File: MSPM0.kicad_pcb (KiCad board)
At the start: 2 copper layers, 0 parts

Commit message: Positioned components, made schematic adjustment accordingly Created ground layer
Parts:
- added C1: 10u, Capacitor_SMD:C_0805_2012Metric, F.Cu at (61.0, 87.8)
- added C10: 10u, Capacitor_SMD:C_0805_2012Metric, F.Cu at (48.0, 80.1)
- added C11: 470n, Capacitor_SMD:C_0603_1608Metric, F.Cu at (51.3, 82.6)
- added C12: 470n, Capacitor_SMD:C_0603_1608Metric, F.Cu at (54.5, 86.1)
- added C13: 470n, Capacitor_SMD:C_0603_1608Metric, F.Cu at (54.5, 91.1)
- added C14: 470n, Capacitor_SMD:C_0603_1608Metric, F.Cu at (70.0, 98.1)
- added C2: 470n, Capacitor_SMD:C_0603_1608Metric, F.Cu at (64.0, 81.8)
- added C3: 470n, Capacitor_SMD:C_0603_1608Metric, F.Cu at (68.5, 81.6)
- added C4: 470n, Capacitor_SMD:C_0603_1608Metric, F.Cu at (76.0, 91.6)
- added C5: 15p, Capacitor_SMD:C_0603_1608Metric, F.Cu at (63.0, 94.9)
- added C6: 15p, Capacitor_SMD:C_0603_1608Metric, F.Cu at (57.0, 94.8)
- added C7: 470n, Capacitor_SMD:C_0603_1608Metric, F.Cu at (43.7, 82.1)
- added C8: 470n, Capacitor_SMD:C_0603_1608Metric, F.Cu at (45.2, 82.1)
- added C9: 10u, Capacitor_SMD:C_0805_2012Metric, F.Cu at (54.8, 80.1)
- added D1: USBLC6-2SC6, Package_TO_SOT_SMD:SOT-23-6, F.Cu at (44.7, 87.3)
- added FID1: Fiducial, Fiducial:Fiducial_1mm_Mask2mm, F.Cu at (42.2, 76.2)
- added FID2: Fiducial, Fiducial:Fiducial_1mm_Mask2mm, F.Cu at (89.9, 76.2)
- added FID3: Fiducial, Fiducial:Fiducial_1mm_Mask2mm, F.Cu at (89.9, 97.8)
- added J1: USB4105-GF-A, Connector_USB:USB_C_Receptacle_GCT_USB4105-xx-A_16P_TopMnt_Horizontal, F.Cu at (36.0, 86.4)
- added J2: TC2030, Connector:Tag-Connect_TC2030-IDC-FP_2x03_P1.27mm_Vertical, F.Cu at (81.5, 88.4)
- added MH1: M3, MountingHole:MountingHole_3.2mm_M3_Pad_Via, F.Cu at (95.2, 97.8)
- added MH2: M3, MountingHole:MountingHole_3.2mm_M3_Pad_Via, F.Cu at (95.2, 76.2)
- added MH3: M3, MountingHole:MountingHole_3.2mm_M3_Pad_Via, F.Cu at (36.8, 97.8)
- added MH4: M3, MountingHole:MountingHole_3.2mm_M3_Pad_Via, F.Cu at (36.8, 76.2)
- added R1: 0R, Capacitor_SMD:C_0603_1608Metric, F.Cu at (68.5, 80.1)
- added R2: 5k1, Capacitor_SMD:C_0603_1608Metric, F.Cu at (74.5, 91.6)
- added R3: 100k, Capacitor_SMD:C_0603_1608Metric, F.Cu at (60.5, 90.3)
- added R4: 0R, Capacitor_SMD:C_0603_1608Metric, F.Cu at (44.5, 84.3)
- added R5: 5k1, Capacitor_SMD:C_0603_1608Metric, F.Cu at (41.0, 92.6)
- added R6: 5k1, Capacitor_SMD:C_0603_1608Metric, F.Cu at (40.8, 79.8)
- added R7: 5k1, Capacitor_SMD:C_0603_1608Metric, F.Cu at (69.5, 95.6)
- added R8: 5k1, Capacitor_SMD:C_0603_1608Metric, F.Cu at (66.5, 95.6)
- added U1: MSPM0G3507SPTR, Package_QFP:LQFP-48_7x7mm_P0.5mm, F.Cu at (67.8, 88.1)
- added U2: SPX3819M5-L-3-3, Package_TO_SOT_SMD:SOT-23-5, F.Cu at (51.3, 80.1)
- added U3: CH340E, Package_SO:MSOP-10_3x3mm_P0.5mm, F.Cu at (54.5, 88.6)
- added U4: LIS2DH, Package_LGA:LGA-14_2x2mm_P0.35mm_LayoutBorder3x4y, F.Cu at (68.0, 98.1)
- added X1: 8MHz, Crystal:Crystal_SMD_3225-4Pin_3.2x2.5mm, F.Cu at (60.0, 94.8)
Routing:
- added copper zone on B.Cu, net GND
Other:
- board outline added: 66 x 29.2 mm

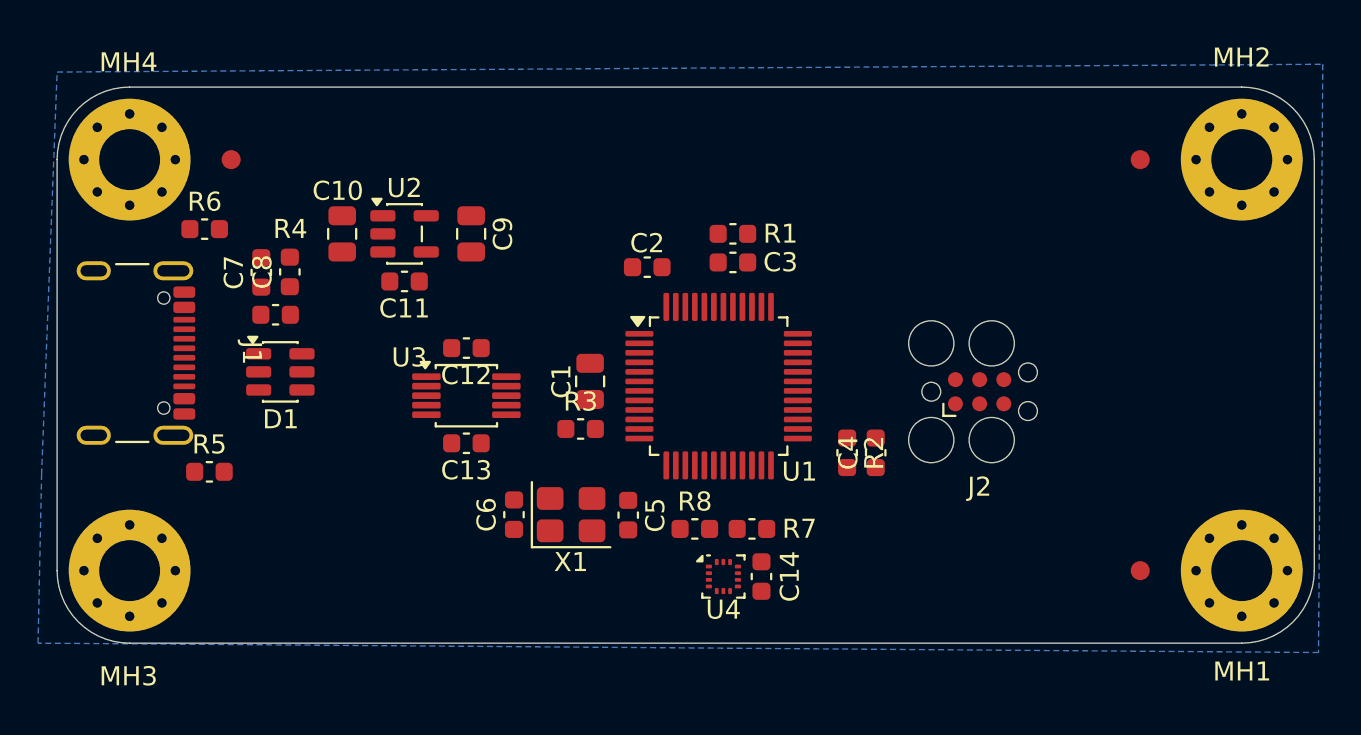
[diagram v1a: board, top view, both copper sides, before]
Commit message: Completed mk. I
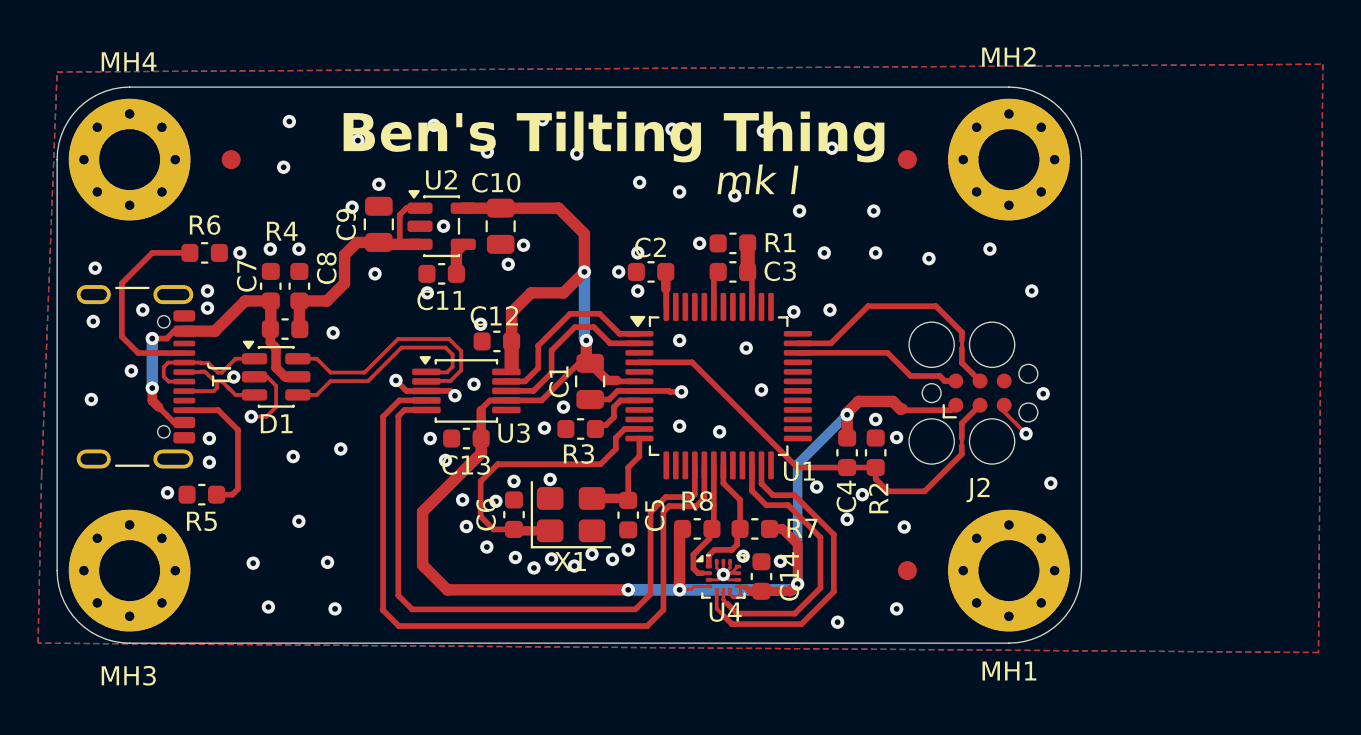
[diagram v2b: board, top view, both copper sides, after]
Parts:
- moved MH1 12.2 mm to (83.0, 97.8)
- moved MH2 12.2 mm to (83.0, 76.2)
- moved FID2 12.2 mm to (77.7, 76.2)
- moved FID3 12.2 mm to (77.7, 97.8)
- moved C10 8.33 mm to (56.3, 79.7)
- moved C9 4.88 mm to (49.9, 79.6), turned to 90 degrees
- moved C11 1.99 mm to (53.2, 82.2)
- moved U2 1.99 mm to (53.2, 79.7)
- moved C12 1.64 mm to (56.1, 85.8)
- moved R5 1.26 mm to (40.6, 93.8), turned to 180 degrees
- moved J1 1.25 mm to (36.0, 87.6)
- moved R6 1.25 mm to (40.8, 81.1)
- moved C8 0.90 mm to (45.7, 82.8)
- moved R4 0.90 mm to (45.0, 85.1)
- moved C7 0.88 mm to (44.2, 82.8)
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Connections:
- D1 pad 1: /USBC_D+ -> /USBC_D-
- D1 pad 3: /USBC_D- -> /USBC_D+
- D1 pad 4: /USB_D- -> /USB_D+
- D1 pad 6: /USB_D+ -> /USB_D-
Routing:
- net +3V3: track 0.00 -> 90.8 mm, vias 0 -> 6
- net /UART0_CTS: track 0.00 -> 37.5 mm
- net /UART0_RTS: track 0.00 -> 33.4 mm
- net /NRST: track 0.00 -> 23.9 mm
- net GND: track 0.00 -> 20.1 mm, vias 0 -> 97
- net +VBUS: track 0.00 -> 17.4 mm, vias 0 -> 2
- net INT2: track 0.00 -> 17.0 mm
- net /HFXIN: track 0.00 -> 15.6 mm
- net INT1: track 0.00 -> 14.9 mm
- net +VBUSF: track 0.00 -> 13.0 mm
- net /SWCLK: track 0.00 -> 12.9 mm
- net /USB_D-: track 0.00 -> 12.9 mm
- net /USB_D+: track 0.00 -> 11.5 mm
- net /USB_CC1: track 0.00 -> 10.7 mm
- net /UART0_TX: track 0.00 -> 9.58 mm
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- added copper zone on F.Cu, net GND
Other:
- board size 66 x 29.2 mm -> 53.8 x 29.2 mm
- board text added: "Ben's Tilting Thing"
- board text added: "mk I"
